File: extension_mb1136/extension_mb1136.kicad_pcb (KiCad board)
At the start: 2 copper layers, 70 x 57.5 mm, 31 parts, among them CN1 Conn_02x19_Odd_Even, CN2 Conn_02x19_Odd_Even, CN3 Conn_01x08, CN4 Conn_01x06, CN5 Conn_01x08, CN6 Conn_01x10, J1 Conn_01x03, J2 Conn_01x03, Q1 S9013, SW1 USB_SEL, SW2 USB_SEL, U1 STMPS2151MTR, U2 USBLC6-2

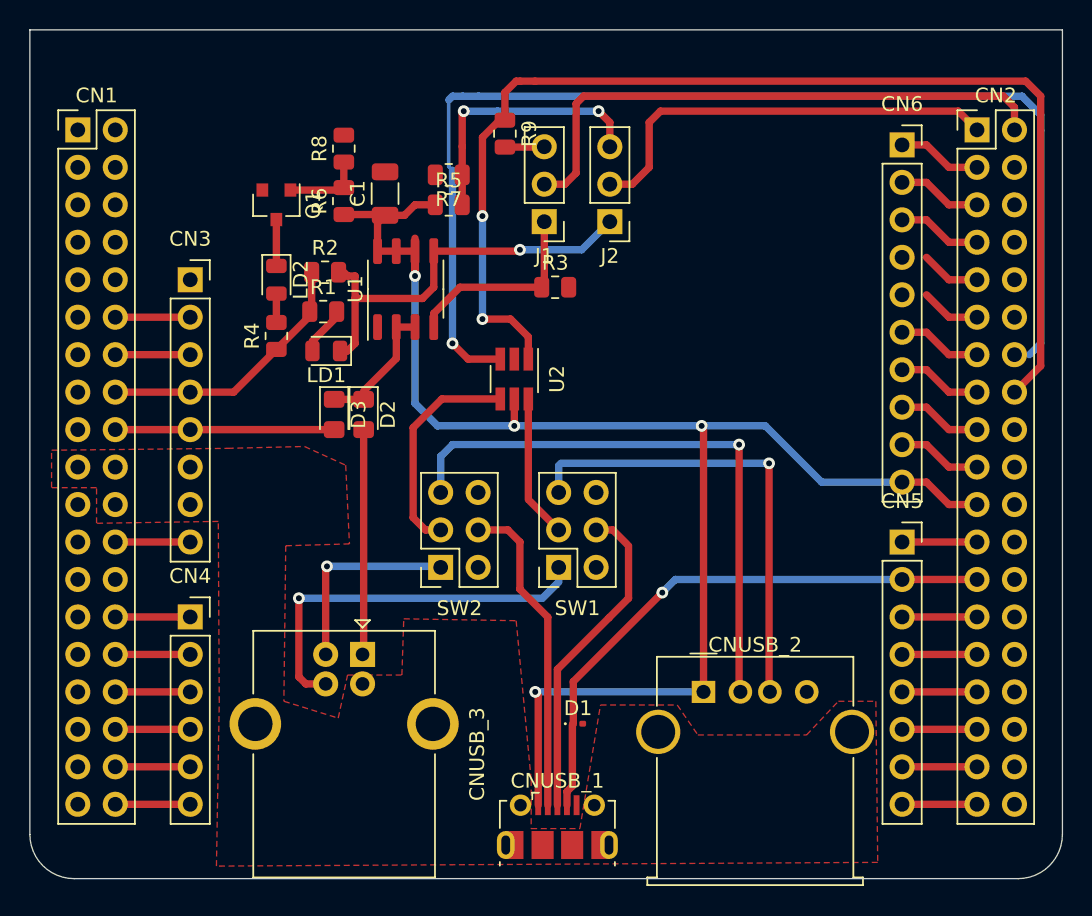
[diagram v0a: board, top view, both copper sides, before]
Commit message: update pcb
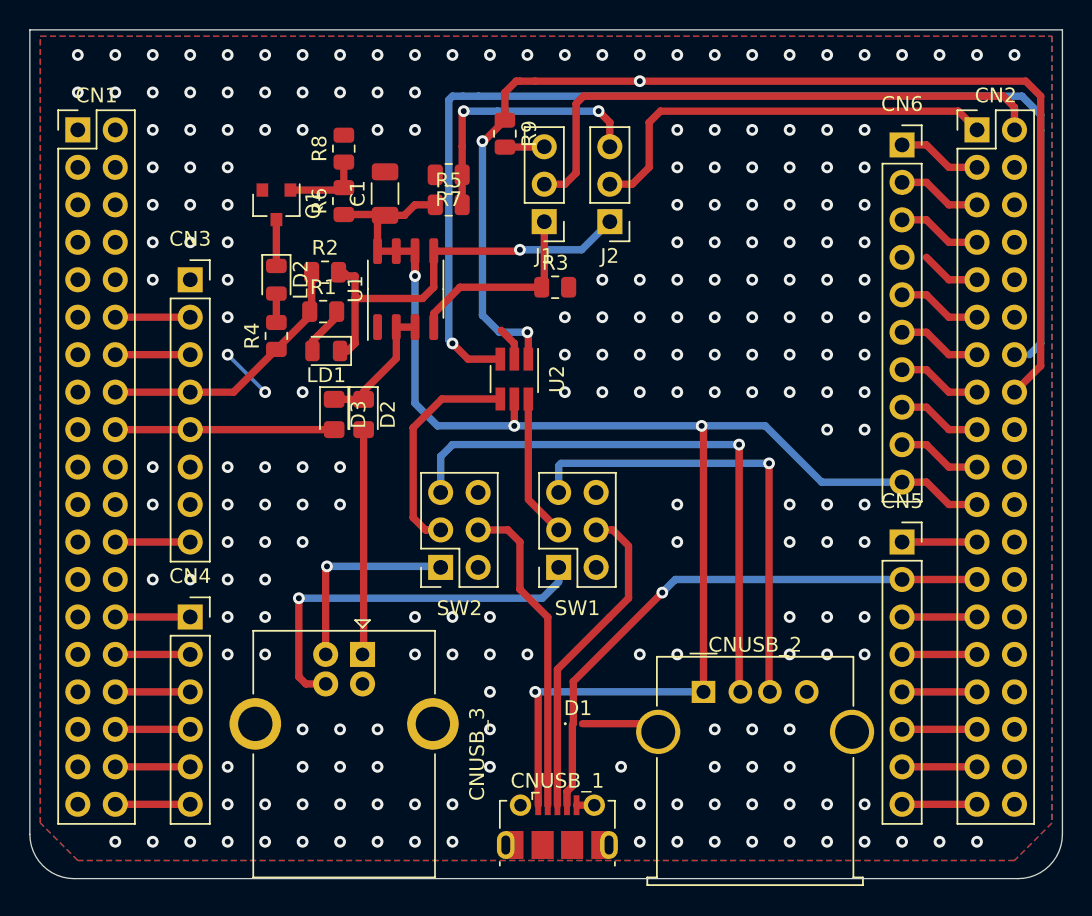
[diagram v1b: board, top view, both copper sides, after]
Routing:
- net GND: track 4.05 -> 16.5 mm, vias 0 -> 214
- net PA5: track 4.05 -> 5.71 mm
- net PA9: track 103.2 -> 102.3 mm
- net PB12: track 79.2 -> 79.4 mm, vias 2 -> 3
- added copper zone on B.Cu, net GND
